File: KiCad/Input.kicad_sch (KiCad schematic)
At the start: 661 parts, among them J1 R_Phono_In, J10 VCC_IN, J11 VCC_OUT, J12 EMK_In, J15 Mic_Effekt_Out, J16 Mic_Effekt_Out, J17 Mic_Effekt_Out, J18 Mic_Effekt_Out, J19 Phono/Line_Out, J2 L_Phono_In, J20 Mic_Effekt_Out, J21 Conn_01x05_bridged, J22 EMK_In, J24 Mic_Effekt_In, J25 Mic_Effekt_In, J26 Phono/Line_In, J27 Mic_Effekt_In, J28 Pegel_Out, J29 Pegel_Out, J3 R_Line_In, J30 Pegel_In, J31 Pegel_In, J32 Pegel_In, J33 Pegel_In, J34 LED_Out, J35 LED_In, J36 VU_Meter_Out, J37 AUX_Send_3, J38 AUX_Send_1, J39 AUX_Send_2, J4 L_Line_In, J40 Bass_Out, J41 Kick_Out, J42 Mid_Out, J43 High_Out, J44 Line_Out_L, J45 Line_Out_R, J5 Mic_In, J6 Effekt_In, J7 AUX_RET_1, J8 AUX_RET_2, J9 AUX_RET_3, SW1 SW_DPST, SW10 SW_SPDT, SW11 SW_SPDT, SW12 SW_SPDT, SW2 SW_SPDT, SW3 SW_SPDT, SW4 SW_SPDT, SW5 SW_SPDT, SW6 SW_SPDT, SW7 SW_SPDT, SW8 SW_SPDT, SW9 SW_Rotary_1x4, U1 TL074, U10 TL074, U11 TL074, U12 TL074, U13 TL074, U14 TL074, U15 TL074, U16 TL074, U17 TL074, U18 TL074, U19 TL074, U2 TL074, U20 TL074, U21 TL074, U22 TL074, U23 TL074, U24 TL074, U25 TL074, U26 TL074, U3 TL074, U4 TL074, U5 TL074, U6 REC10K-2409, U7 REC10K-2415, U8 TL074, U9 TL074

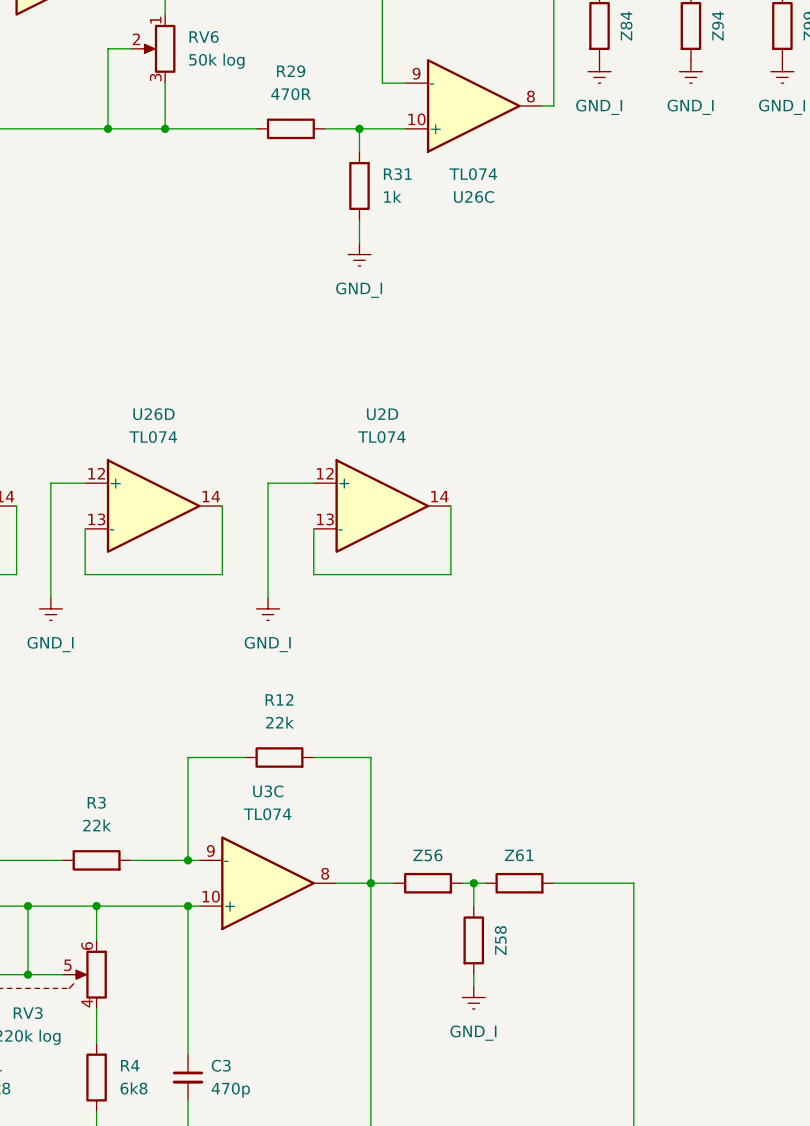
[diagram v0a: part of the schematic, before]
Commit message: PCB Update
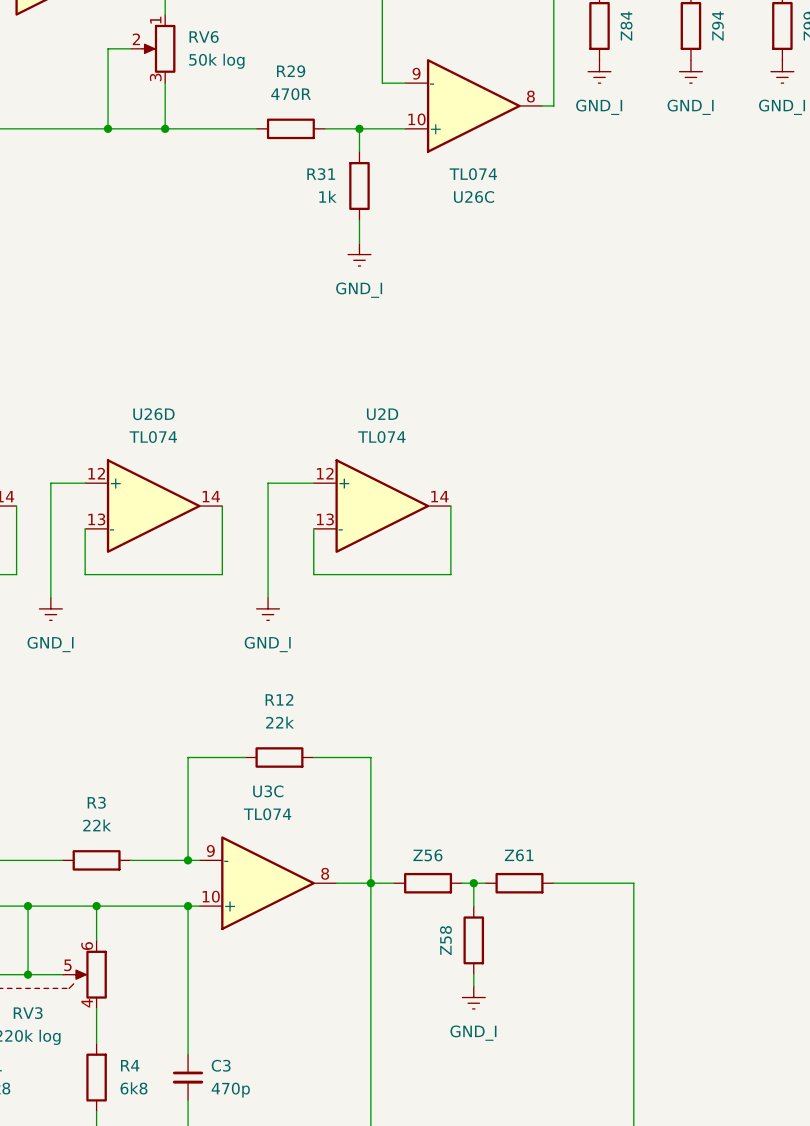
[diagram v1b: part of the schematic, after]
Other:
- moved on the sheet: R31
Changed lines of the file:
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@@
 	(symbol
 		(lib_id "Device:R")
-		(at 210.82 135.89 180)
+		(at 210.82 135.89 0)
+		(mirror x)
 		(unit 1)
 		(exclude_from_sim no)
@@
 		(on_board yes)
 		(dnp no)
-		(fields_autoplaced yes)
 		(property "Reference" "R31"
-			(at 213.36 134.6199 0)
+			(at 208.28 134.6199 0)
 			(effects
 				(font
@@
 		)
 		(property "Value" "1k"
-			(at 213.36 137.1599 0)
+			(at 208.28 137.1599 0)
 			(effects
 				(font
@@
 		)
 		(property "Footprint" "Resistor_SMD:R_0805_2012Metric_Pad1.20x1.40mm_HandSolder"
-			(at 212.598 135.89 90)
+			(at 209.042 135.89 90)
 			(effects
 				(font
@@
 		(lib_id "Device:R")
 		(at 223.52 219.71 0)
+		(mirror y)
 		(unit 1)
 		(exclude_from_sim no)
@@
 		(dnp no)
 		(property "Reference" "Z58"
-			(at 226.568 219.71 90)
+			(at 220.472 219.71 90)
 			(effects
 				(font
@@
 		)
 		(property "Value" "~"
-			(at 227.33 219.71 90)
+			(at 219.71 219.71 90)
 			(effects
 				(font
@@
 		)
 		(property "Footprint" "Resistor_SMD:R_0805_2012Metric_Pad1.20x1.40mm_HandSolder"
-			(at 221.742 219.71 90)
+			(at 225.298 219.71 90)
 			(effects
 				(font

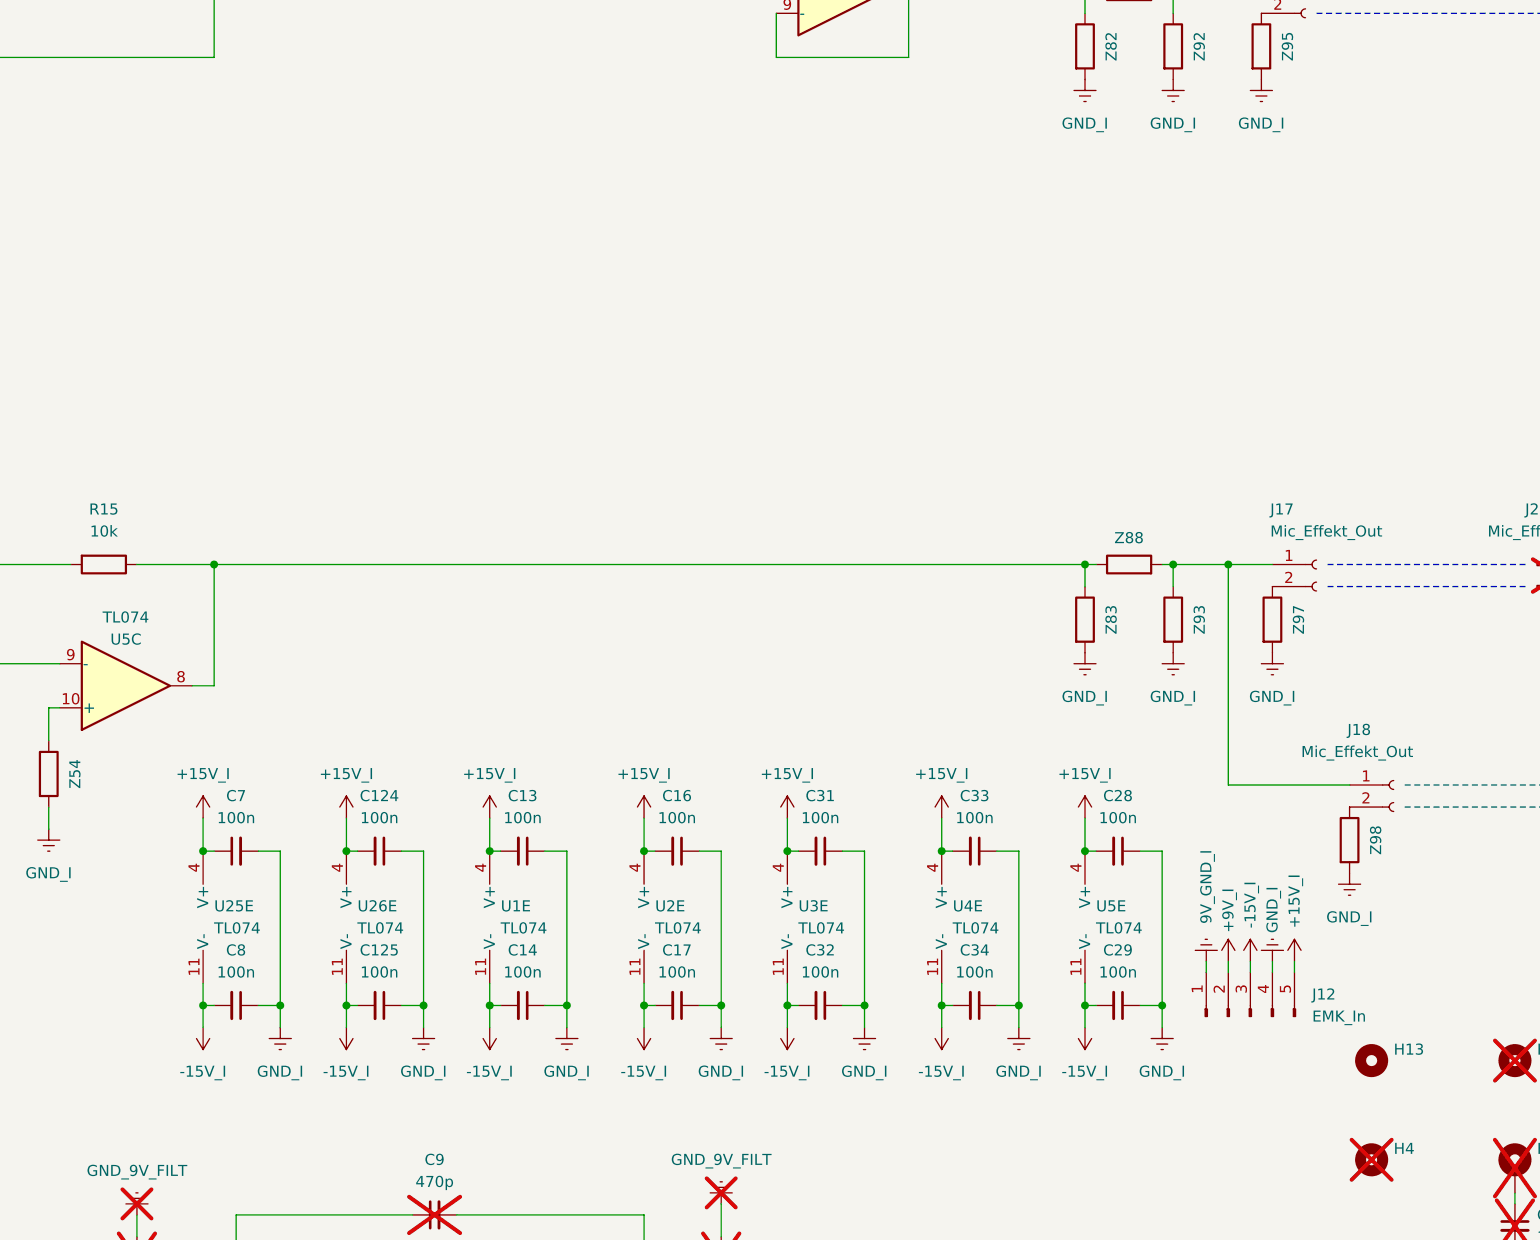
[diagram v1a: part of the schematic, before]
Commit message: PCB Final Update
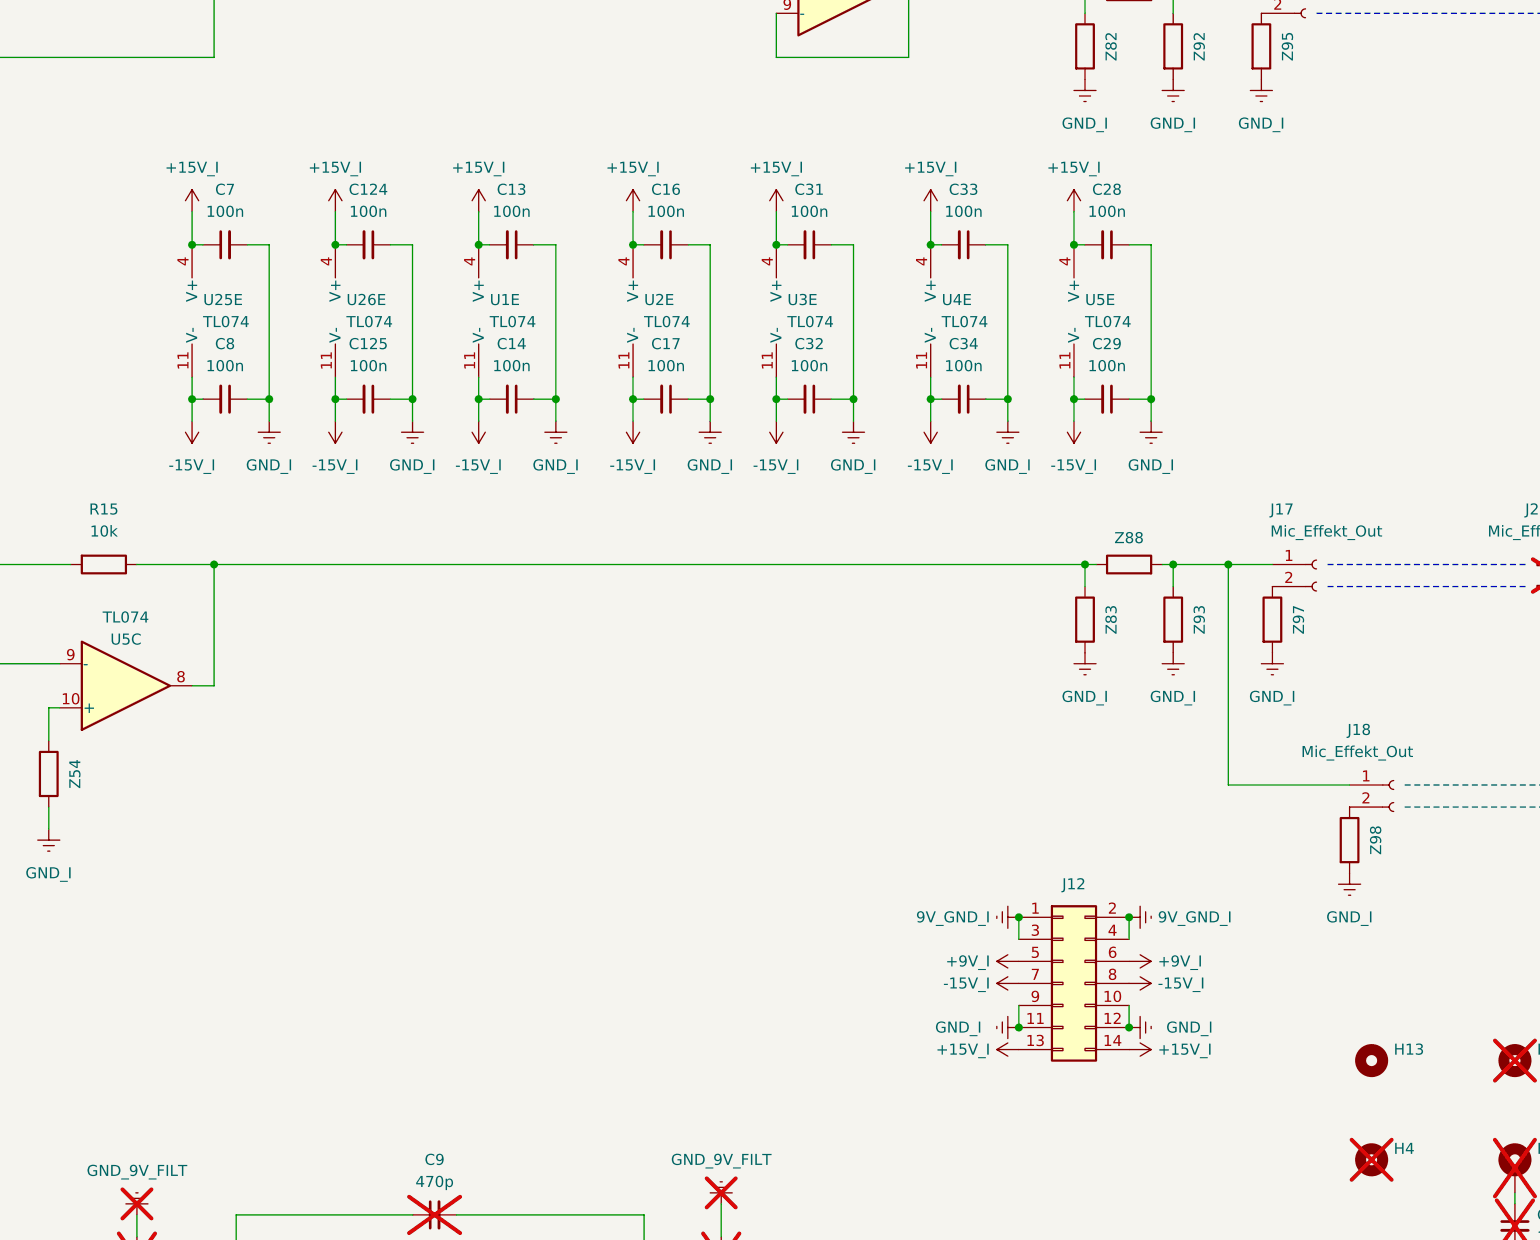
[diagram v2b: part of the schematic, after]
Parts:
- removed J12: EMK_In, Connector_PinHeader_2.54mm_LongPads:PinHeader_1x05_P2.54mm_Vertical_LongPads, symbol Connector:Conn_01x05_Pin
- added J12: Conn_02x07_Odd_Even, Connector_PinHeader_2.54mm:PinHeader_2x07_P2.54mm_Vertical, symbol Connector_Generic:Conn_02x07_Odd_Even
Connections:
- net +15V_I: now also J12.13 (Pin_13), J12.14 (Pin_14)
- net +9V_I: now also J12.5 (Pin_5), J12.6 (Pin_6)
- net -15V_I: now also J12.7 (Pin_7), J12.8 (Pin_8)
- net 9V_GND_I: now also J12.1 (Pin_1), J12.2 (Pin_2), J12.3 (Pin_3), J12.4 (Pin_4)
- net GND_I: now also J12.10 (Pin_10), J12.11 (Pin_11), J12.12 (Pin_12), J12.9 (Pin_9)
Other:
- moved on the sheet: C124, C125, C13, C14, C16, C17, C28, C29, C31, C32, C33, C34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
